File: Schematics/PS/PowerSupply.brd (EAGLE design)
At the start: 158.8 x 110.7 mm, 79 parts, among them IC1 LM317MABDT, IC2 LM337, T1 IRFP240, T2 IRFP240

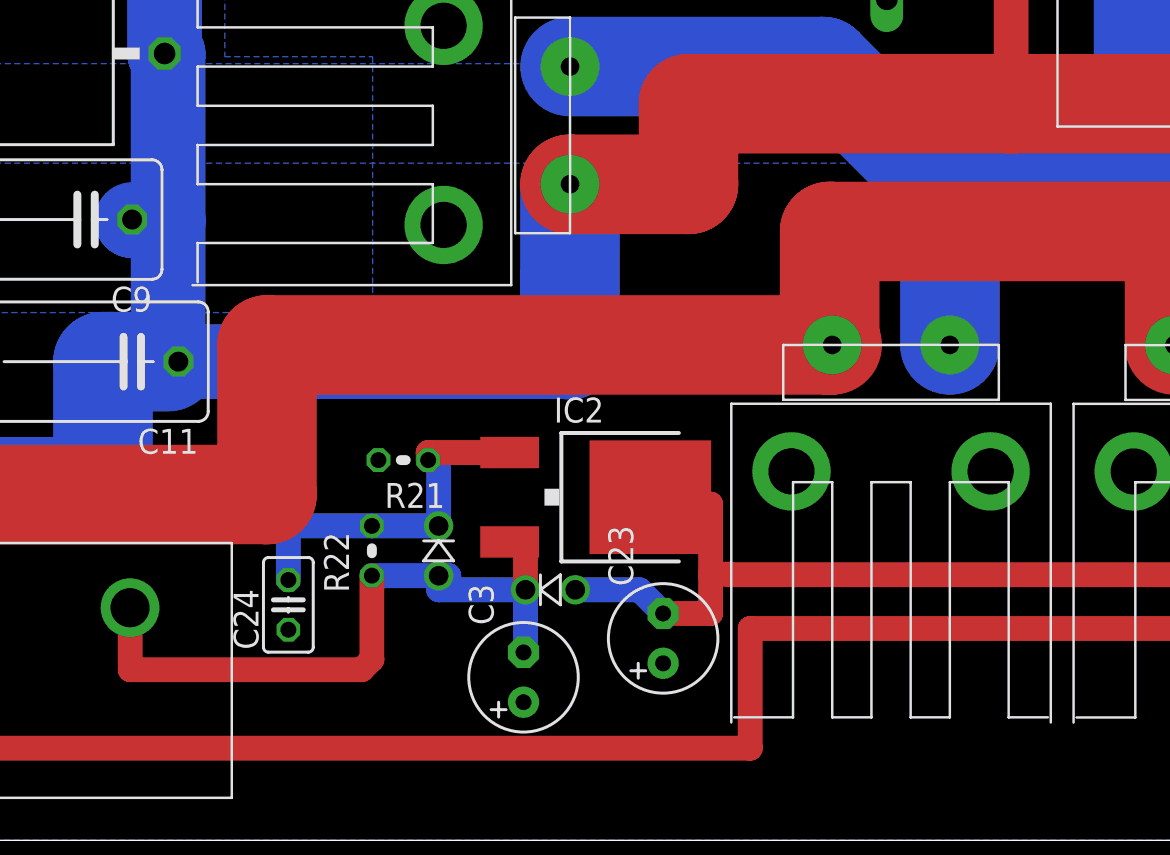
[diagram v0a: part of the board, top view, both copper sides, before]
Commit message: updates to PS layout
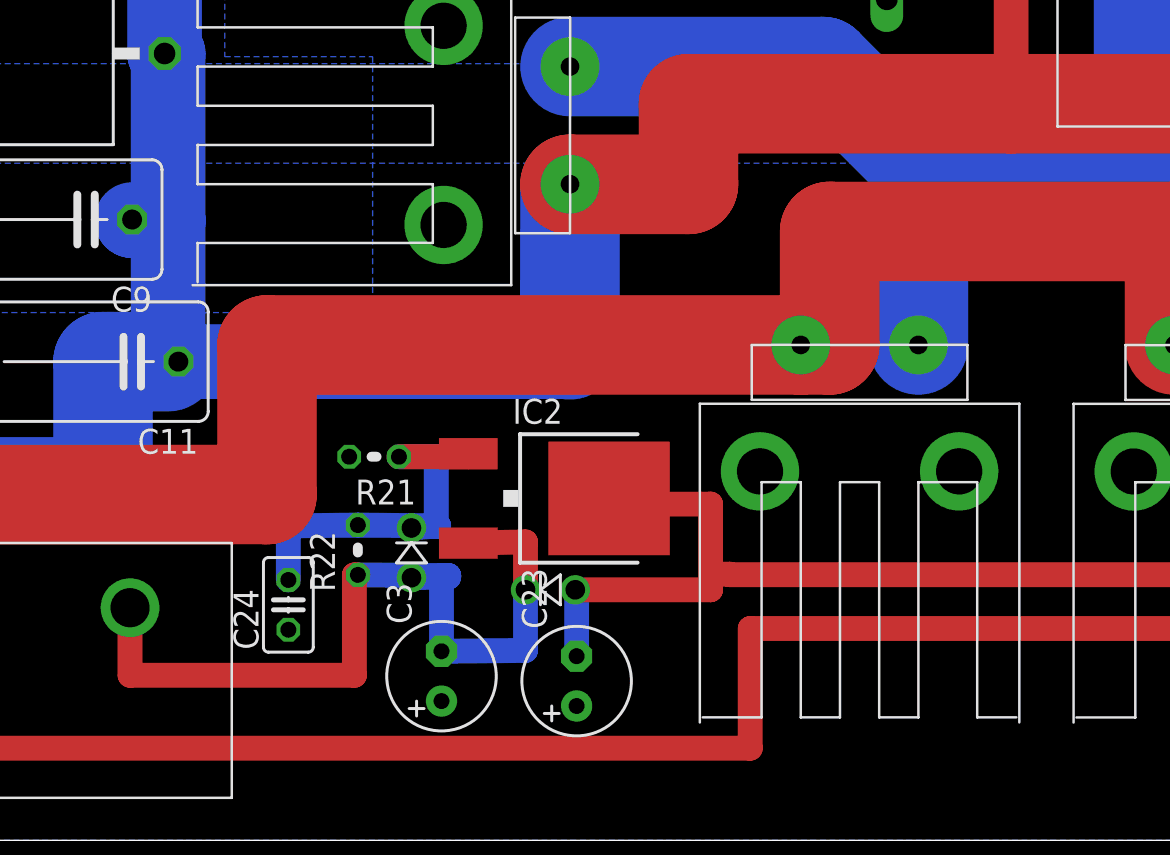
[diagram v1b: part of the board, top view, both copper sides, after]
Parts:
- moved C23 4.92 mm to (71.8, 24.4)
- moved C3 4.19 mm to (64.9, 24.6)
- moved IC2 2.11 mm to (71.1, 33.7)
- moved D8 1.61 mm to (86.2, 41.5)
- moved R21 1.50 mm to (61.5, 35.8)
- moved D17 1.39 mm to (63.4, 33.7)
- moved R22 0.72 mm to (60.6, 31.1)
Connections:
- net N$15 renamed LINE
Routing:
- net V15-: track 36.2 -> 43.8 mm
- net N$3: track 18.9 -> 21.1 mm
- net V-15UN: track 122.5 -> 124.4 mm
- net VAC+40: track 56.4 -> 57.7 mm
